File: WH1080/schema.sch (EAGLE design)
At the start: 18 parts

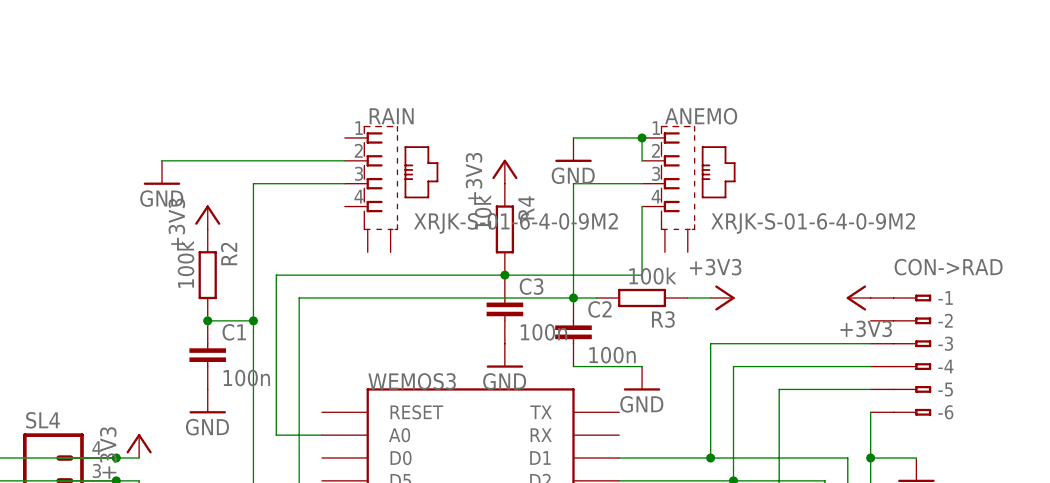
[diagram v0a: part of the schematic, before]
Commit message: +
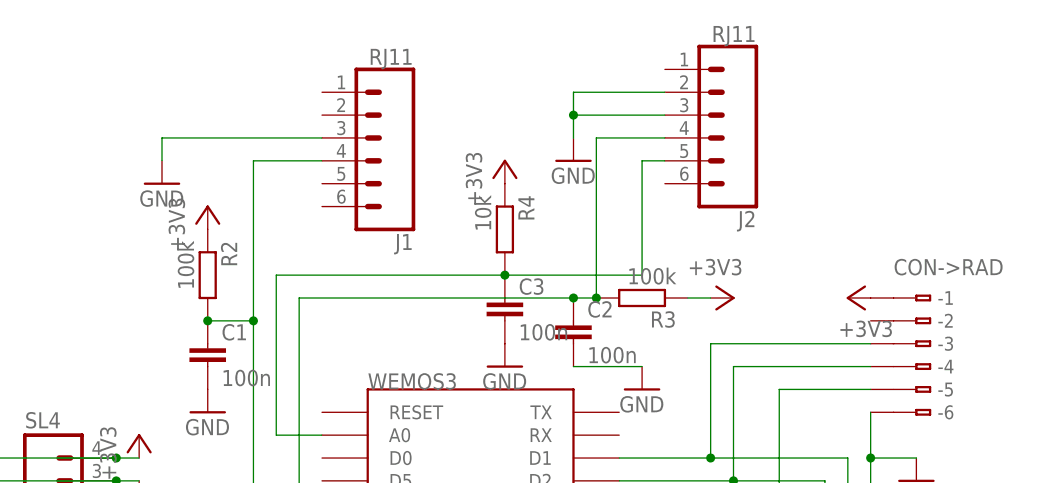
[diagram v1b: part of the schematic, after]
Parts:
- removed ANEMO, RAIN: XRJK-S-01-6-4-0-9M2, con-xmultiple:XRJK-S-01-6-4-0-9M2
- added J1, J2: RJ11, SparkFun-Connectors:RJ11-6
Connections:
- net GND: now also J1.3, J2.2, J2.3; no longer ANEMO.1, ANEMO.2, RAIN.2
- net N$1: now also J1.4; no longer RAIN.3
- net N$2: now also J2.5; no longer ANEMO.4
- net N$4: now also J2.4; no longer ANEMO.3
